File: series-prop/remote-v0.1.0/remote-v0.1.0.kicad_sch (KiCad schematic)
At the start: 65 parts, among them IC1 LM66200DRLR, J1 Conn_01x17, J10 Conn_01x03_Pin, J11 Conn_01x04_Pin, J13 USB_C_Receptacle_USB2.0_16P, J2 Conn_01x04_Pin, J4 Conn_01x17, J5 Conn_01x01_Pin, J6 Screw_Terminal_01x02, J7 Screw_Terminal_01x03, J8 Conn_Coaxial, J9 SM04B-SRSS-TB, SW1 SW_Push, SW2 SW_Push, SW3 SW_Push, SW4 SW_Push, U1 RT9080-33GJ5, U2 W25Q16JVS, U3 RP2040, U4 RFM69HCW, U5 AP63205WU, U6 74AHCT1G125, U7 3544-2, Y1 Crystal_GND24

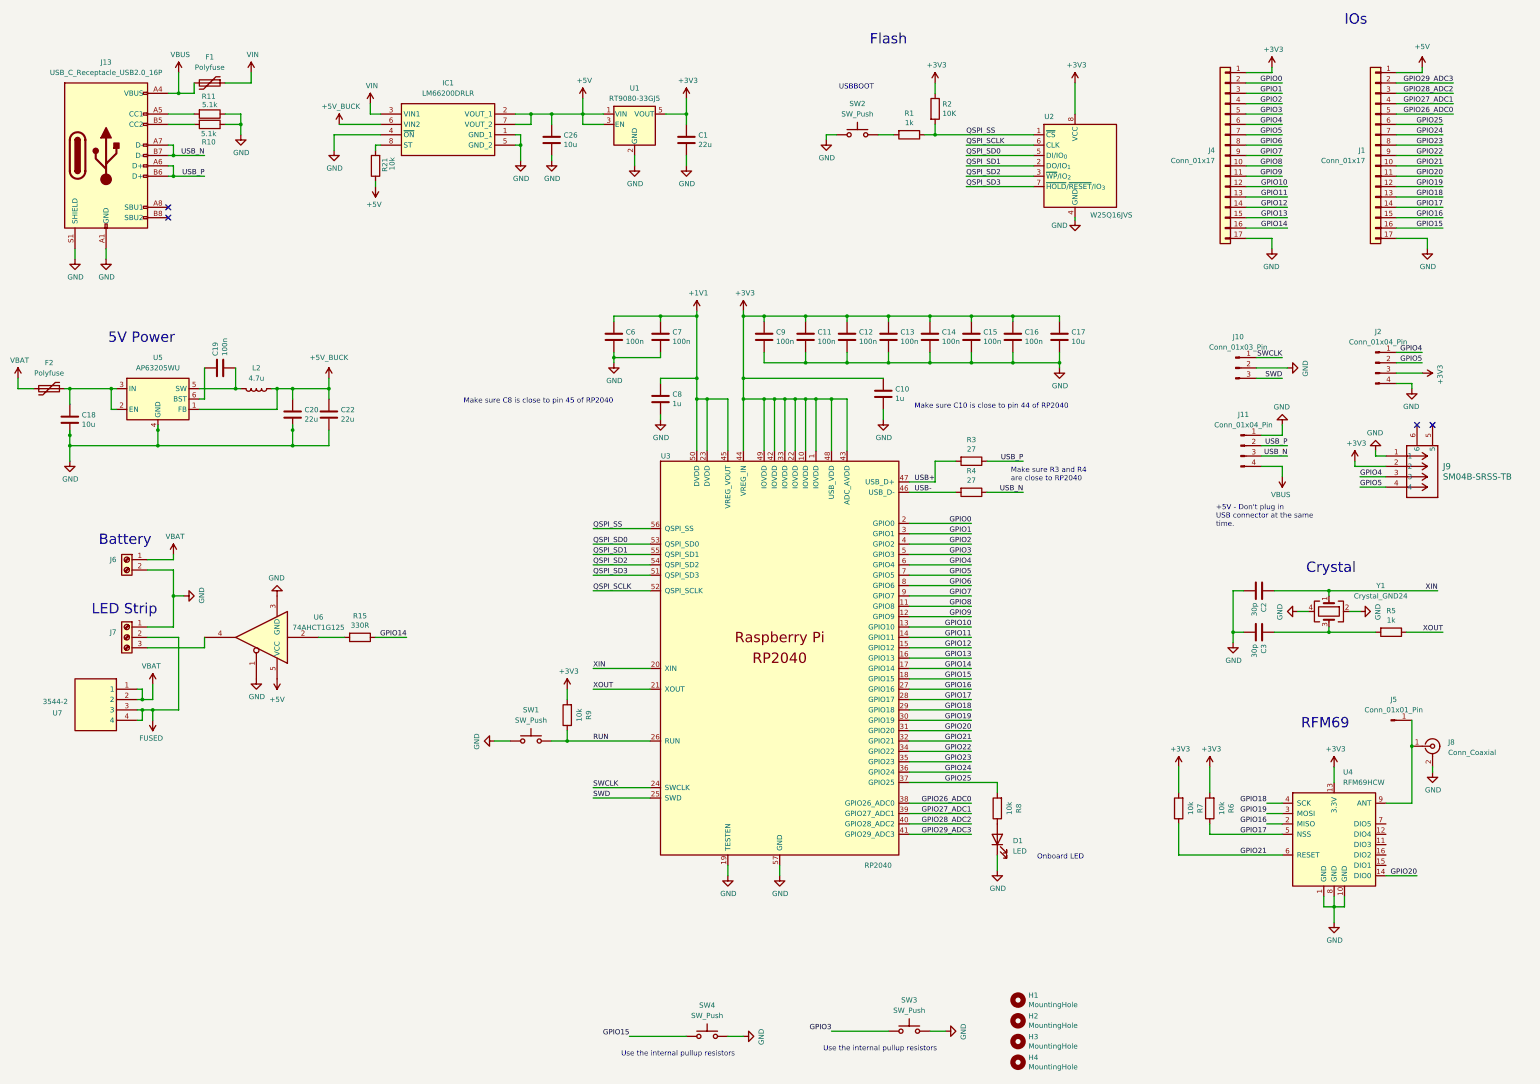
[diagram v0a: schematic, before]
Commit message: added remote design files
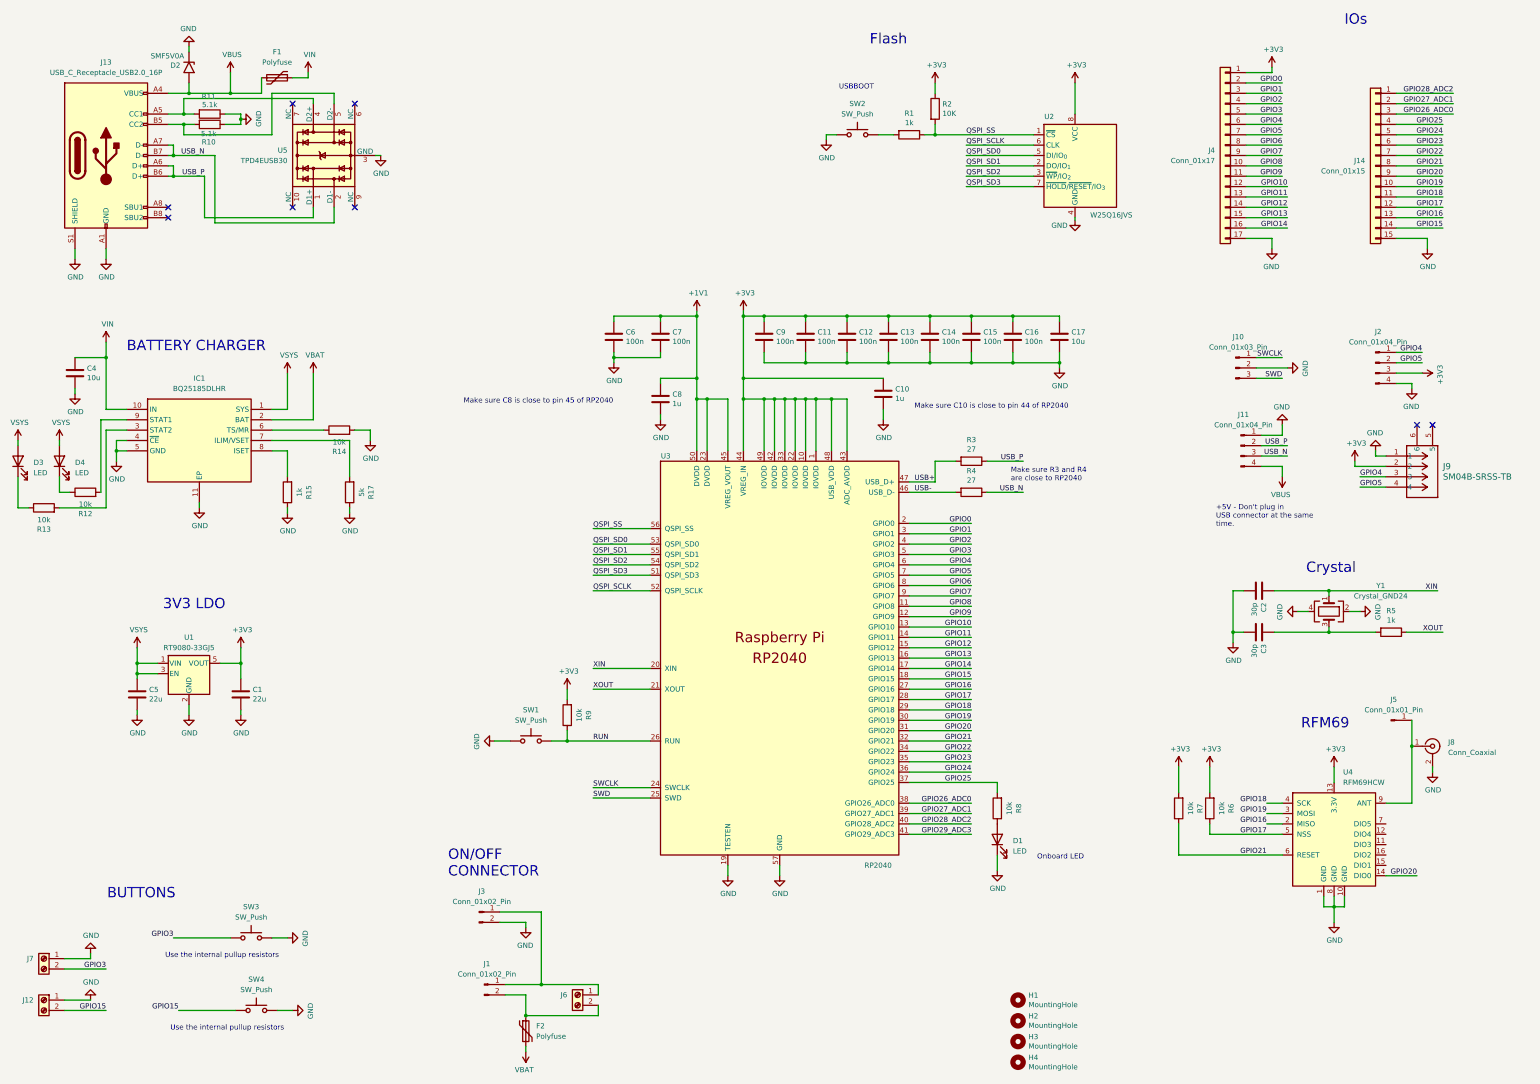
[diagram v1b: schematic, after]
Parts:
- removed C18, C26: 10u, Capacitor_SMD:C_1206_3216Metric, symbol Device:C
- removed C19: 100n, Capacitor_SMD:C_0603_1608Metric, symbol Device:C
- removed C20, C22: 22u, Capacitor_SMD:C_0805_2012Metric, symbol Device:C
- removed IC1: LM66200DRLR, PicoLume:LM66200DRLR, symbol LM66200DRLR:LM66200DRLR
- removed J1: Conn_01x17, Connector_PinHeader_2.54mm:PinHeader_1x17_P2.54mm_Vertical, symbol Connector_Generic:Conn_01x17
- removed J7: Screw_Terminal_01x03, TerminalBlock:TerminalBlock_bornier-3_P5.08mm, symbol Connector:Screw_Terminal_01x03
- removed L2: 4.7u, Inductor_SMD:L_Sunlord_SWPA4030S, symbol Device:L
- removed R21: 10k, Resistor_SMD:R_0603_1608Metric, symbol Device:R
- removed U5: AP63205WU, Package_TO_SOT_SMD:TSOT-23-6, symbol Regulator_Switching:AP63203WU
- removed U6: 74AHCT1G125, Package_TO_SOT_SMD:SOT-23-5, symbol 74xGxx:74AHCT1G125
- removed U7: 3544-2, PicoLume:3544-2, symbol PicoLume:3544-2
- added C4: 10u, Capacitor_SMD:C_0603_1608Metric, symbol Device:C
- added C5: 22u, Capacitor_SMD:C_0805_2012Metric, symbol Device:C
- added D2: SMF5V0A, Diode_SMD:D_SMF, symbol Diode:SMF5V0A
- added D3, D4: LED, LED_SMD:LED_0603_1608Metric, symbol Device:LED
- added IC1: BQ25185DLHR, PicoLume:SON40P220X200X80-11N, symbol PicoLume:BQ25185DLHR
- added J1: Conn_01x02_Pin, Connector_PinHeader_2.54mm:PinHeader_1x02_P2.54mm_Vertical, symbol Connector:Conn_01x02_Pin
- added J12, J7: Screw_Terminal_01x02, TerminalBlock:TerminalBlock_bornier-2_P5.08mm, symbol Connector:Screw_Terminal_01x02
- added J14: Conn_01x15, Connector_PinHeader_2.54mm:PinHeader_1x15_P2.54mm_Vertical, symbol Connector_Generic:Conn_01x15
- added J3: Conn_01x02_Pin, Connector_JST:JST_PH_S2B-PH-K_1x02_P2.00mm_Horizontal, symbol Connector:Conn_01x02_Pin
- added R12, R13, R14: 10k, Resistor_SMD:R_0603_1608Metric, symbol Device:R
- added R17: 5k, Resistor_SMD:R_0603_1608Metric, symbol Device:R
- added U5: TPD4EUSB30, Package_SON:USON-10_2.5x1.0mm_P0.5mm, symbol Power_Protection:TPD4EUSB30
- R15: value 330R -> 1k; LCSC C23138 -> C21190
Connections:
- net GND: now also R15.1, C4.2, C5.2, D2.1 (A1), IC1.11 (EP), IC1.4 (~{CE}), IC1.5 (GND), J12.1 (Pin_1), J14.15 (Pin_15), J3.2 (Pin_2), J7.1 (Pin_1), R14.2, R17.1, U5.3 (GND), U5.8 (GND); no longer J6.2 (Pin_2)
- net GPIO14: no longer R15.1
- net GPIO15: now also J12.2 (Pin_2), J14.14 (Pin_14)
- net GPIO16: now also J14.13 (Pin_13)
- net GPIO17: now also J14.12 (Pin_12)
- net GPIO18: now also J14.11 (Pin_11)
- net GPIO19: now also J14.10 (Pin_10)
- net GPIO20: now also J14.9 (Pin_9)
- net GPIO21: now also J14.8 (Pin_8)
- net GPIO22: now also J14.7 (Pin_7)
- net GPIO23: now also J14.6 (Pin_6)
- net GPIO24: now also J14.5 (Pin_5)
- net GPIO25: now also J14.4 (Pin_4)
- net GPIO26_ADC0: now also J14.3 (Pin_3)
- net GPIO27_ADC1: now also J14.2 (Pin_2)
- net GPIO28_ADC2: now also J14.1 (Pin_1)
- net GPIO3: now also J7.2 (Pin_2)
- net USB_N: now also U5.2 (D1-)
- net USB_P: now also U5.1 (D1+)
- net VBAT: now also IC1.2 (BAT); no longer J6.1 (Pin_1)
- net VBUS: now also D2.2 (A2)
- net VIN: now also C4.1, IC1.10 (IN)
- net at R15.2: now also IC1.8 (ISET)
- net at J13.B5 (CC2), R10.2: now also U5.5 (D2-)
- net at F2.1: now also J6.2 (Pin_2), J1.2 (Pin_2)
- net at J13.A5 (CC1), R11.2: now also U5.4 (D2+)
- net +5V renamed VSYS
- net VSYS: now also C5.1, D3.2 (A), D4.2 (A), IC1.1 (SYS)
- new net: D4.1 (K), R12.1
- new net: IC1.9 (STAT1), R12.2
- new net: J1.1 (Pin_1), J3.1 (Pin_1), J6.1 (Pin_1)
- new net: IC1.6 (TS/MR), R14.1
- new net: IC1.3 (STAT2), R13.2
- new net: IC1.7 (ILIM/VSET), R17.2
- new net: D3.1 (K), R13.1
- no-connect marks 4 -> 8
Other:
- note added: "3V3 LDO"
- note added: "BATTERY CHARGER"
- note added: "BUTTONS"
- note added: "ON/OFF CONNECTOR"
- note removed: "5V Power"
- note removed: "Battery"
- note removed: "LED Strip"
- moved on the sheet: C1, F1, J6, SW3, SW4, U1
